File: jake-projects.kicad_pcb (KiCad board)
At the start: 2 copper layers, 26 x 25.5 mm, 12 parts, among them J1 Conn_01x02_Pin, SW1 ;-;, SW2 SW_Push, SW4 SW_SPST, U2 ATtiny85-20P

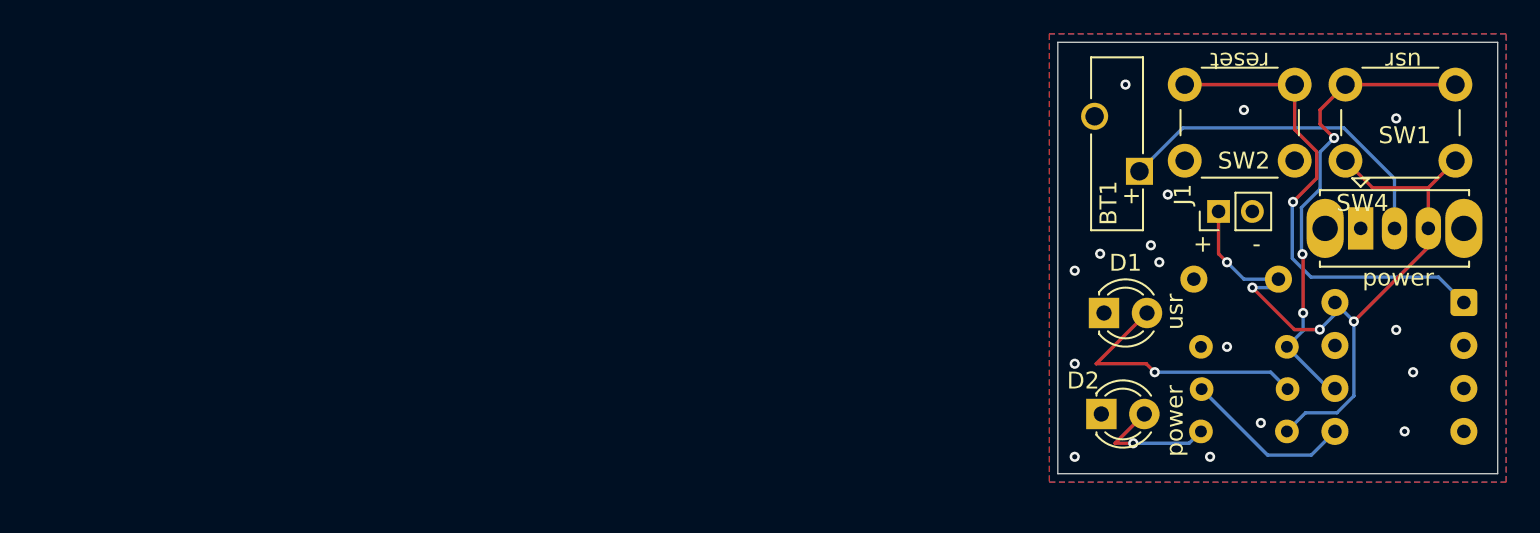
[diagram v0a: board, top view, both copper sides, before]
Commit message: revised/final draft of schematic + pcb
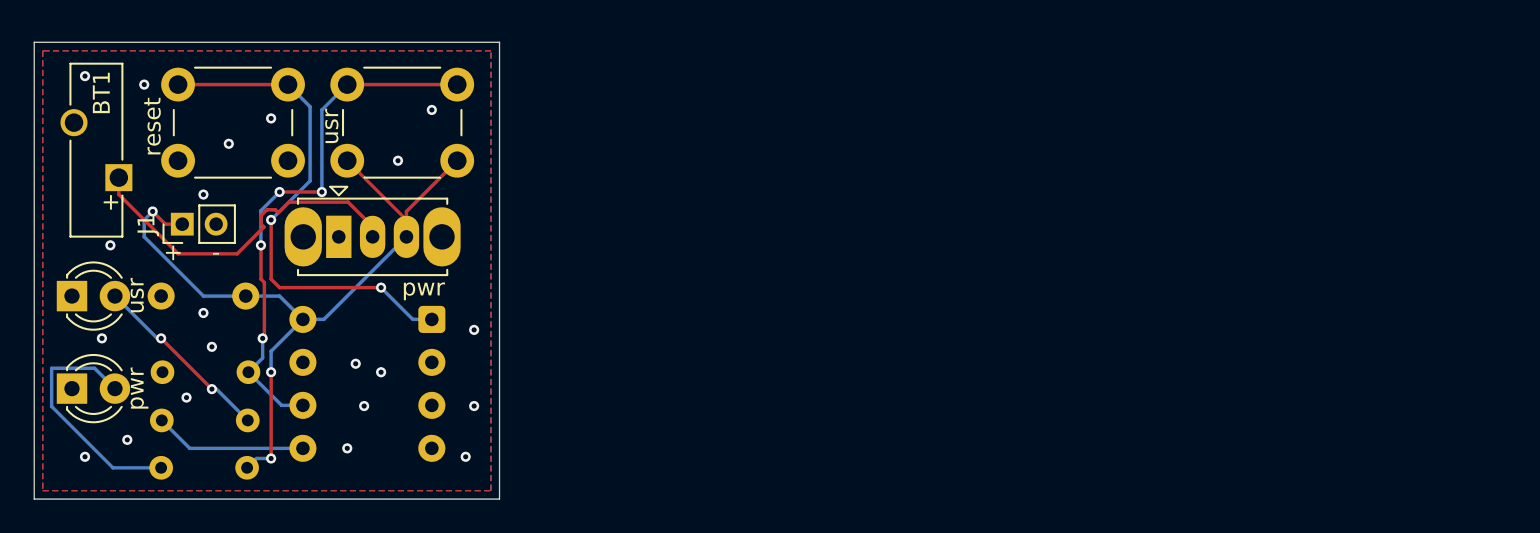
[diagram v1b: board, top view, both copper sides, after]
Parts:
- removed D1: ;-;, LED_THT:LED_D3.0mm
- removed D2: LED, LED_THT:LED_D3.0mm
- removed SW1: ;-;, Button_Switch_THT:SW_PUSH_6mm_H7.3mm
- removed SW2: SW_Push, Button_Switch_THT:SW_PUSH_6mm_H7.3mm
- removed SW4: SW_SPST, Button_Switch_THT:SW_Slide_SPDT_Straight_CK_OS102011MS2Q
- added pwr: pwr, Button_Switch_THT:SW_Slide_SPDT_Straight_CK_OS102011MS2Q, F.Cu at (123.0, 98.0)
- added pwr: pwr, LED_THT:LED_D3.0mm, F.Cu at (107.2, 107.0)
- added reset: reset, Button_Switch_THT:SW_PUSH_6mm_H7.3mm, F.Cu at (113.5, 89.0)
- added usr: usr, LED_THT:LED_D3.0mm, F.Cu at (107.2, 101.5)
- added usr: usr, Button_Switch_THT:SW_PUSH_6mm_H7.3mm, F.Cu at (123.5, 89.0)
- J1: value Conn_01x02_Pin -> Pins
- U2: footprint Package_DIP:DIP-8_W7.62mm -> Package_DIP:DIP-8_W7.62mm_Socket
- moved R3 61.5 mm to (117.6, 111.7)
- moved R1 61.5 mm to (117.6, 108.8)
- moved R2 61.4 mm to (117.7, 106.0)
- moved J1 61.3 mm to (113.8, 97.2)
- moved C1 61.0 mm to (117.5, 101.5)
- moved U2 61.0 mm to (128.5, 102.9)
- moved BT1 60.3 mm to (110.0, 94.5)
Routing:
- net Net-(D2-A): track 7.81 -> 14.5 mm, vias 1 -> 0
- net Net-(D1-A): track 16.2 -> 11.4 mm, vias 1 -> 2
- net Net-(U2-PB1): track 28.1 -> 31.6 mm, vias 3 -> 4
- net VCC: track 43.8 -> 45.6 mm, vias 4 -> 3
- net Net-(U2-AREF/PB0): track 10.1 -> 9.02 mm
- net Net-(U2-~{RESET}/PB5): track 29.1 -> 30.0 mm, vias 1 -> 2
- net GND: vias 16 -> 21
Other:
- board size 26 x 25.5 mm -> 27.5 x 27 mm
- board text removed: "power"
- board text removed: "reset"
- board text removed: "usr"
